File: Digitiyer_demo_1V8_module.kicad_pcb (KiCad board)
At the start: 2 copper layers, 35 x 35 mm, 93 parts, among them J1 Conn_01x08, J2 Conn_01x24, Q1 AO3400A, Q2 SI1308EDL, U1 Opamp_Quad, U2 LM27762DSSR, U3 TMUX1108PWR, U4 RF-BM-ND05, U5 TPS63900DSKR, U6 TXB0108PWR, U8 74LVC1G34GW

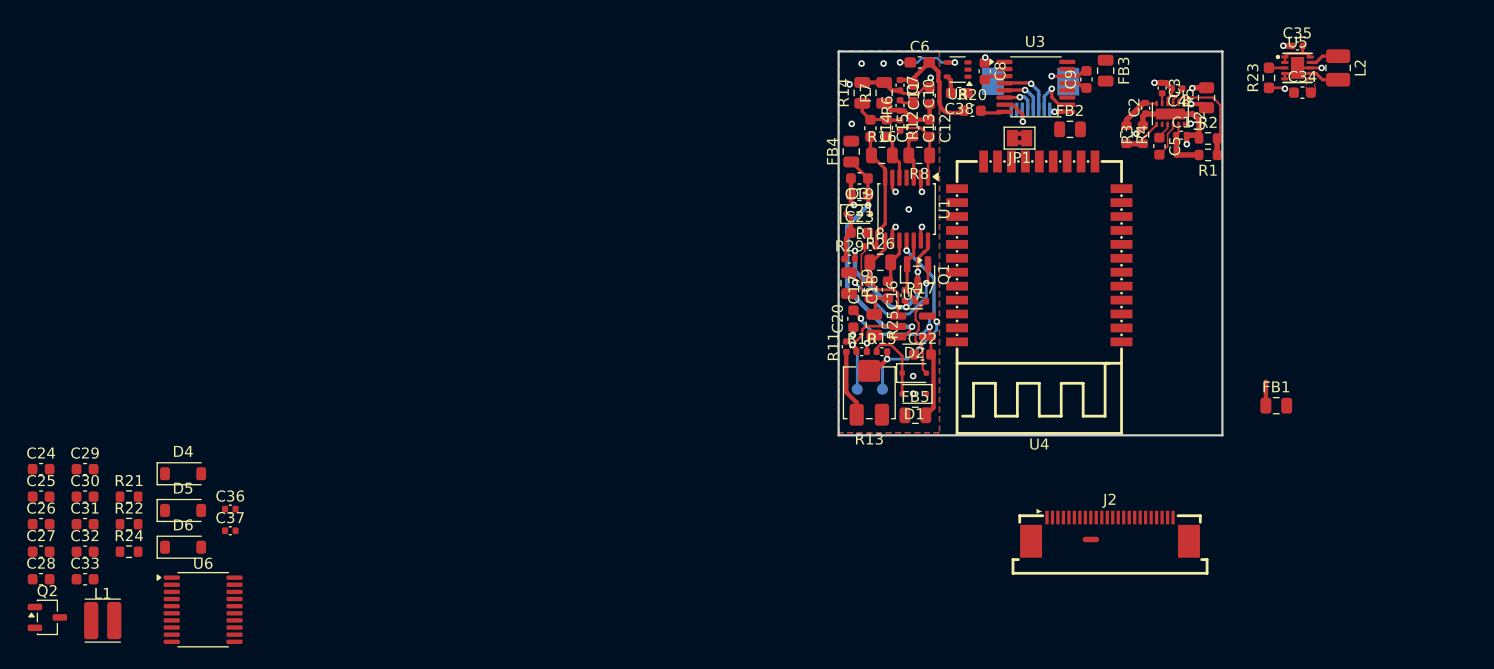
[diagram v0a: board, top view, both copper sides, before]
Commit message: aktualizace
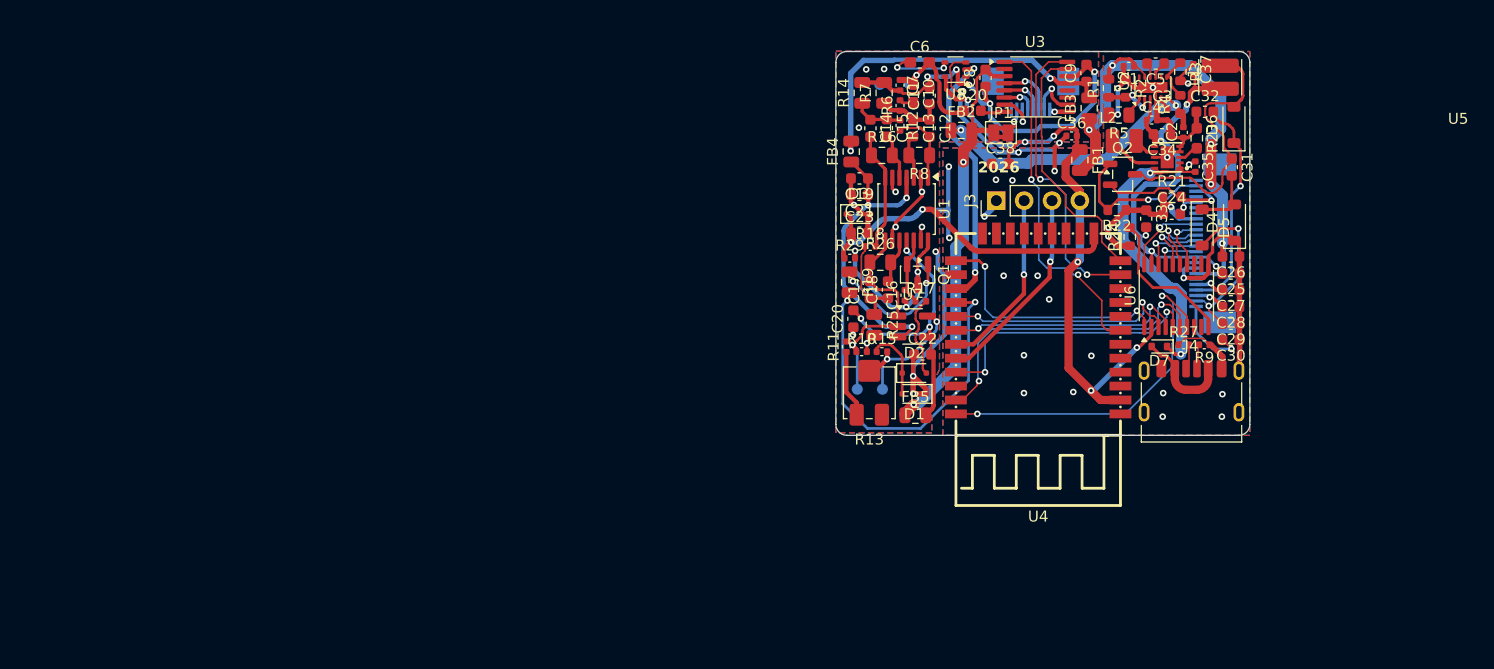
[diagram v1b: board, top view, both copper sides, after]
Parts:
- added D7: LESD5Z5_0T1G, Diode_SMD:D_SOD-523, F.Cu at (181.2, 92.9)
- added J3: Conn_01x04_Pin, Connector_PinHeader_2.54mm:PinHeader_1x04_P2.54mm_Vertical, F.Cu at (166.4, 79.6)
- added J4: USB_C_Receptacle_PowerOnly_6P, Connector_USB:USB_C_Receptacle_HRO_TYPE-C-31-M-17, F.Cu at (184.2, 98.1)
- added R27: 5.1k, Capacitor_SMD:C_0402_1005Metric, F.Cu at (183.5, 92.8)
- added R9: 5.1k, Capacitor_SMD:C_0402_1005Metric, F.Cu at (185.3, 92.7)
- added REF**: TestPoint_Pad_D1.0mm, TestPoint:TestPoint_Pad_D1.0mm, B.Cu at (158.4, 69.0)
- added REF**: TestPoint_Pad_D1.0mm, TestPoint:TestPoint_Pad_D1.0mm, B.Cu at (155.8, 69.0)
- J2, NT1: moved to B.Cu
- moved L1 113.3 mm to (186.8, 68.3), turned to 90 degrees
- moved C28 111.3 mm to (187.8, 89.3), turned to 180 degrees
- moved C26 111.2 mm to (187.8, 84.7), turned to 180 degrees
- moved C27 111.1 mm to (187.8, 87.8), turned to 180 degrees
- moved C25 110.4 mm to (187.8, 86.2), turned to 180 degrees
- moved C32 109.7 mm to (185.4, 71.5)
- moved C31 109.5 mm to (187.8, 76.5), turned to -90 degrees
- moved Q2 106.1 mm to (177.9, 77.2)
- moved C24 105.7 mm to (182.4, 80.8)
- moved C30 105.5 mm to (187.8, 92.3), turned to 180 degrees
- moved C29 105.3 mm to (187.8, 90.8), turned to 180 degrees
- moved D6 103.3 mm to (188.1, 72.7), turned to 90 degrees
- moved C33 102.2 mm to (180.1, 81.2), turned to -90 degrees
- moved R21 99.0 mm to (182.4, 79.2)
- moved D4 98.6 mm to (188.1, 81.6), turned to 90 degrees
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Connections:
- C23 pad 1: /AFE/INTG -> INTG
- D3 pad 1: /AFE/INTG -> INTG
- J2 pad 1: /NC -> unconnected-(J2-Pin_1-Pad1)
- J2 pad 4: /NC -> unconnected-(J2-Pin_4-Pad4)
- R29 pad 1: /AFE/INTG -> INTG
- U4 pad 13: /AIN0 -> INTG
- U4 pad 28: unconnected-(U4-SWDIO-Pad28) -> /SWDIO
- U4 pad 29: unconnected-(U4-SWCLK-Pad29) -> /SWCLK
- U6 pad 1: /SDI_1V8 -> /BUSY_1V8
- U6 pad 14: /BUSY -> /RES
- U6 pad 15: /RES -> /D/C
- U6 pad 16: /D/C -> /CS
- U6 pad 17: /CS -> /SDI
- U6 pad 20: /SDI -> /BUSY
- U6 pad 4: /CS_1V8 -> /SDI_1V8
- U6 pad 5: /D/C_1V8 -> /CS_1V8
- U6 pad 6: /RES_1V8 -> /D/C_1V8
- U6 pad 7: /BUSY_1V8 -> /RES_1V8
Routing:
- net GND: track 22.2 -> 98.3 mm, vias 7 -> 30
- net +1V8: track 3.84 -> 57.7 mm, vias 0 -> 6
- net VSSA: track 21.4 -> 74.2 mm, vias 17 -> 18
- net VDD: track 4.94 -> 49.6 mm, vias 0 -> 5
- net +3V3: track 1.72 -> 39.9 mm, vias 0 -> 5
- net VEE: track 1.45 -> 38.8 mm, vias 0 -> 2
- net DISCHARGE: track 0.00 -> 33.7 mm, vias 0 -> 2
- net /RES_1V8: track 0.00 -> 32.7 mm, vias 0 -> 2
- net /A0: track 0.00 -> 31.9 mm, vias 0 -> 2
- net INTG: track 0.00 -> 31.3 mm, vias 0 -> 2
- net VDDA: track 2.25 -> 32.5 mm, vias 0 -> 2
- net /D/C_1V8: track 0.00 -> 28.7 mm, vias 0 -> 2
- net /A1: track 0.00 -> 27.5 mm, vias 0 -> 2
- net Net-(D6-A): track 0.00 -> 26.9 mm
- net /CS_1V8: track 0.00 -> 25.2 mm, vias 0 -> 2
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- added copper zone on B.Cu, net GND
- added copper zone on F.Cu, net GND
- removed copper zone on F.Cu, net +3V3
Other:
- board size 35 x 35 mm -> 37.8 x 35 mm
- board text added: "1V8"
- board text added: "2026"
- board text added: "AFE"
- board text added: "GND"
- board text added: "Prototyp 1: test EMR+EPD Robin Josef Šafařík, 2026"
- board text added: "SWCLK"
- board text added: "SWDIO"
- board text added: "VSSA"

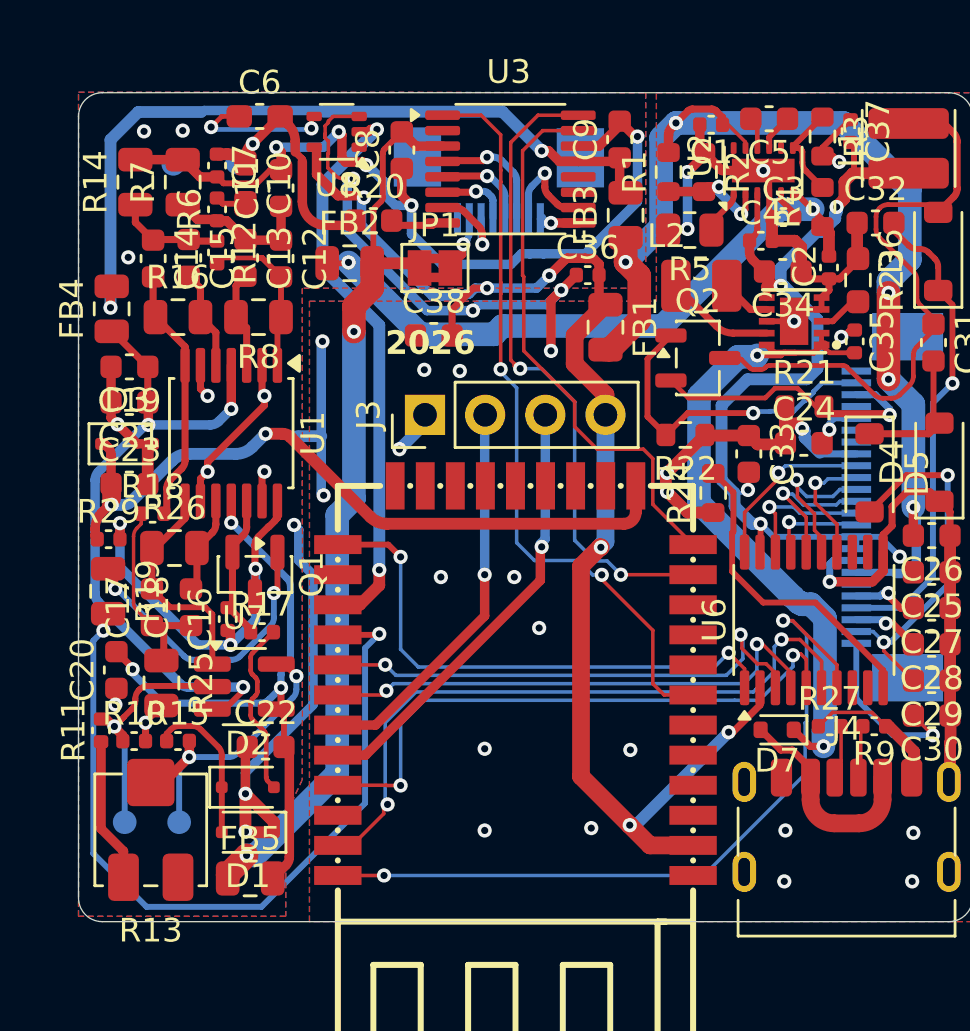
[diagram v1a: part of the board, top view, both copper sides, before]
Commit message: uložení
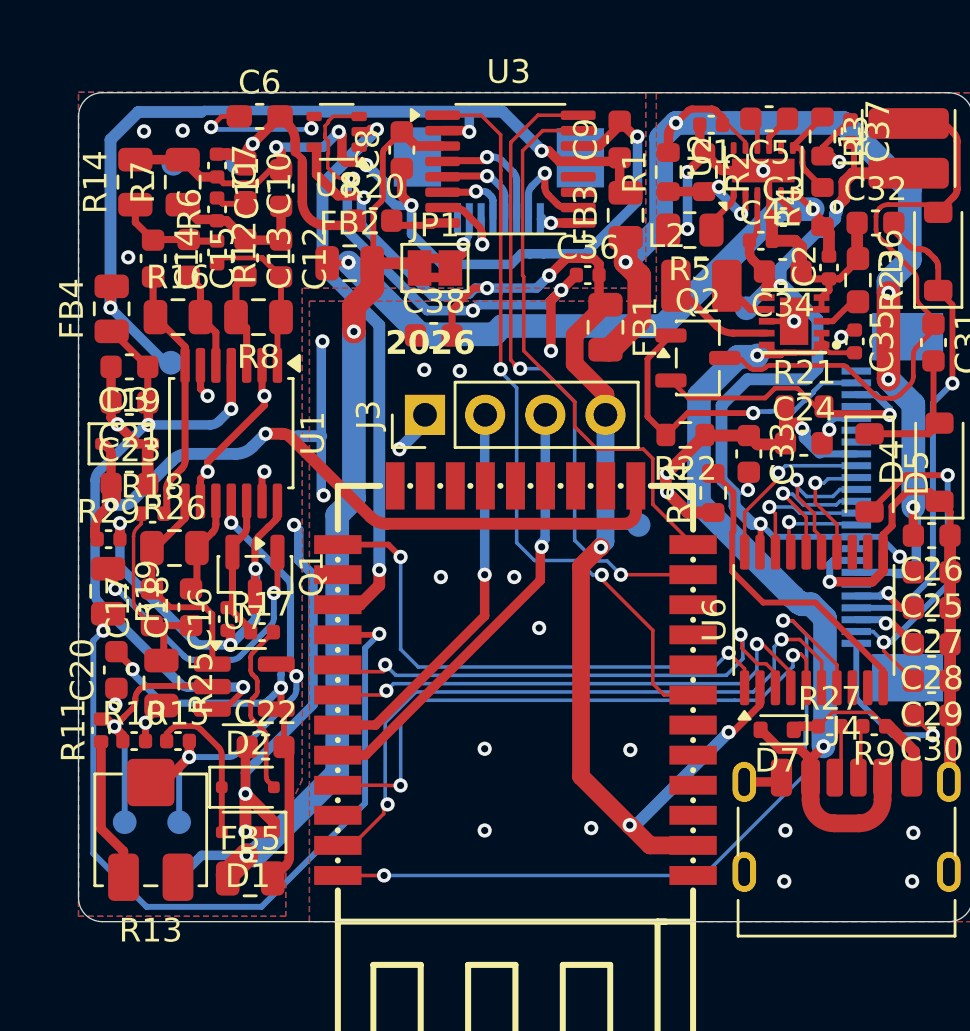
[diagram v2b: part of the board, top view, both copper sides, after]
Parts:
- added REF**: TestPoint_Pad_D1.0mm, TestPoint:TestPoint_Pad_D1.0mm, B.Cu at (175.4, 84.2)
- added REF**: TestPoint_Pad_D1.0mm, TestPoint:TestPoint_Pad_D1.0mm, B.Cu at (179.9, 75.1)
- added REF**: TestPoint_Pad_D1.0mm, TestPoint:TestPoint_Pad_D1.0mm, B.Cu at (155.7, 77.4)
- added REF**: TestPoint_Pad_D1.0mm, TestPoint:TestPoint_Pad_D1.0mm, B.Cu at (156.1, 99.1)
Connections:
- C35 pad 2: Net-(D7-C) -> Net-(D7-A)
- D7 pad 1: Net-(D7-C) -> GND
- U3 pad 2: /EN -> VDDA
- U5 pad 1: Net-(D7-C) -> Net-(D7-A)
- U5 pad 10: Net-(D7-C) -> Net-(D7-A)
- U5 pad 2: Net-(D7-C) -> Net-(D7-A)
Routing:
- net Net-(D7-A): track 10.6 -> 39.7 mm, vias 0 -> 2
- net Net-(D7-C): track 28.5 -> 0.00 mm, vias 2 -> 0
- net VDDA: track 32.5 -> 38.0 mm, vias 2 -> 3
- net VEE: track 38.8 -> 42.0 mm
- net GND: track 98.3 -> 101.0 mm
- net +3V3: track 39.9 -> 41.7 mm
- net +1V8: track 57.7 -> 59.1 mm
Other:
- board text added: "3V3"
- board text added: "Trim"
- board text added: "VDDA"
- board text added: "VEE"
- board text removed: "Prototyp 1: test EMR+EPD Robin Josef Šafařík, 2026"
